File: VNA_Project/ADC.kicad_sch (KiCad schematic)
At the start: 27 parts, among them U3 AD9238BSTZ-20, U4 LT1813CS8-TRPBF, U5 LT1813CS8-TRPBF

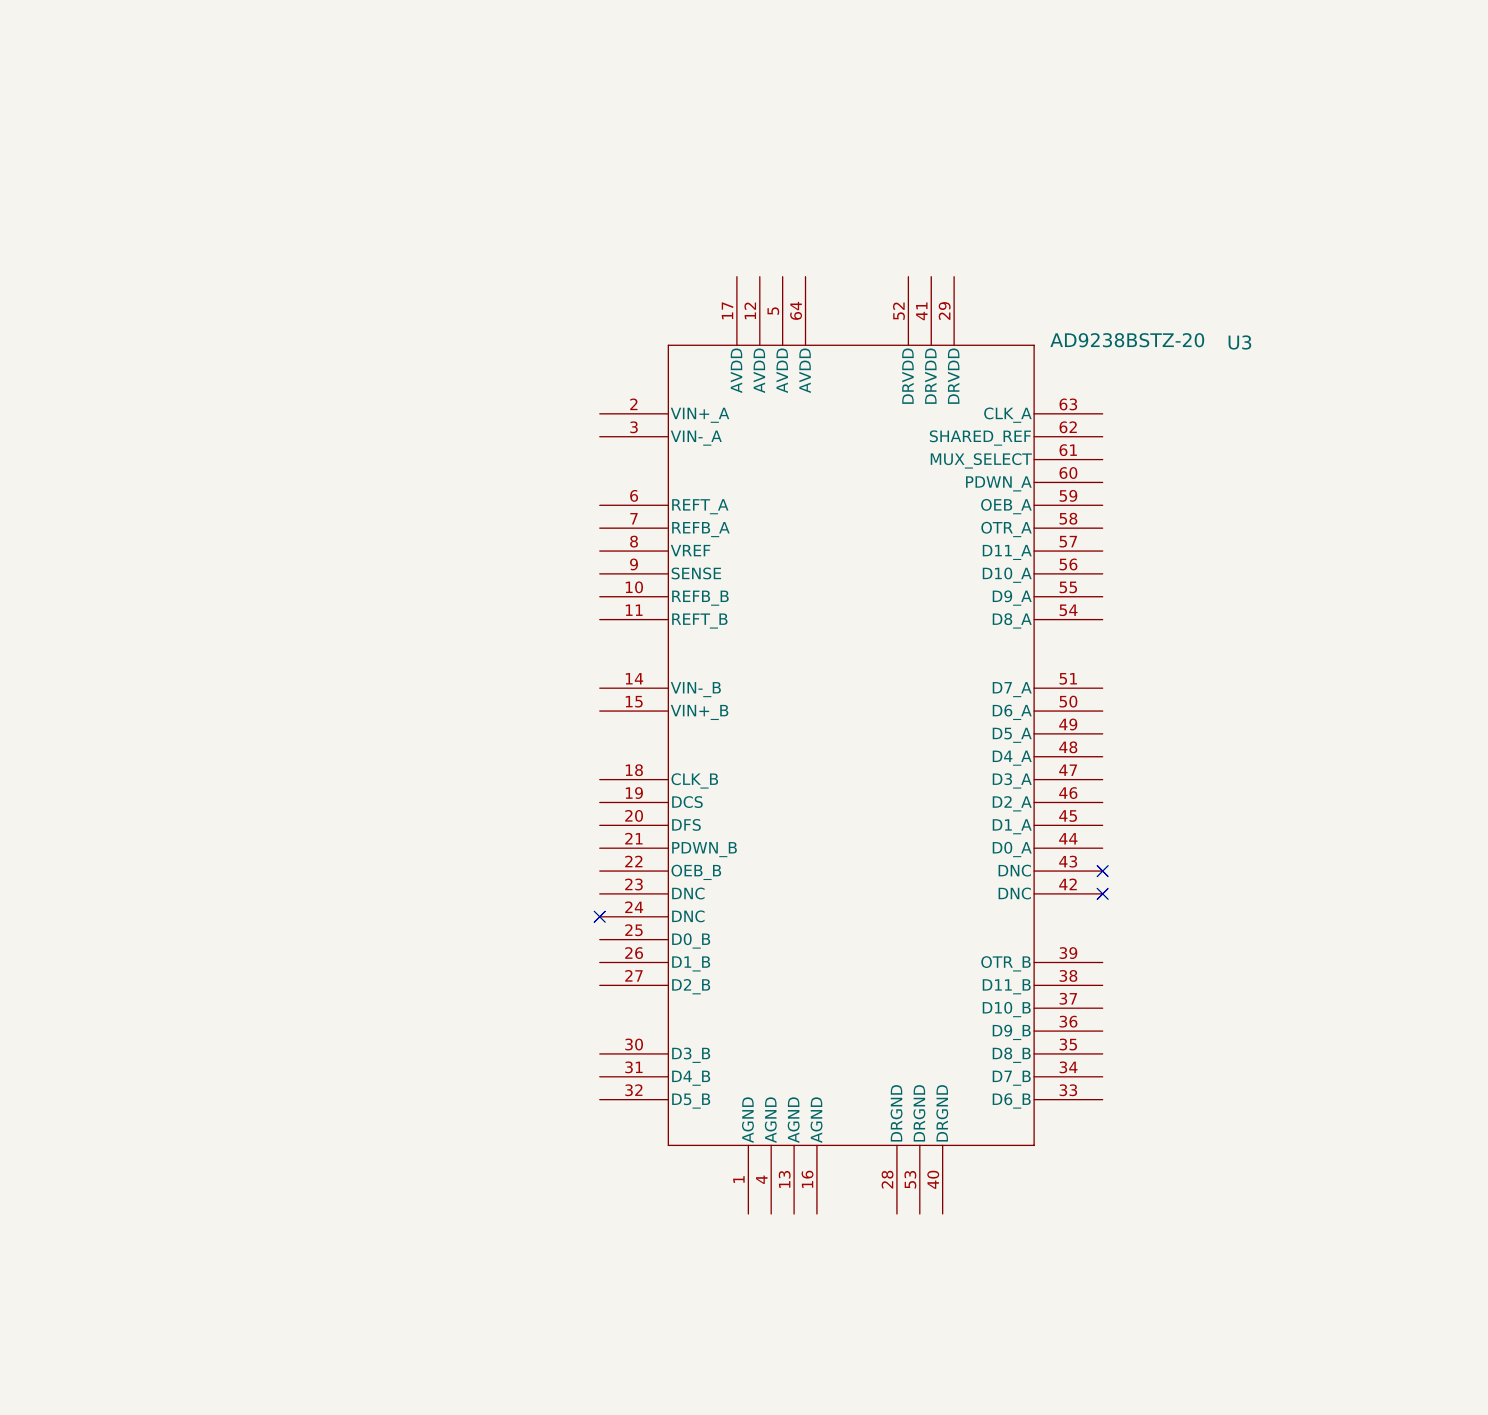
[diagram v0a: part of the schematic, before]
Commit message: adc
adc
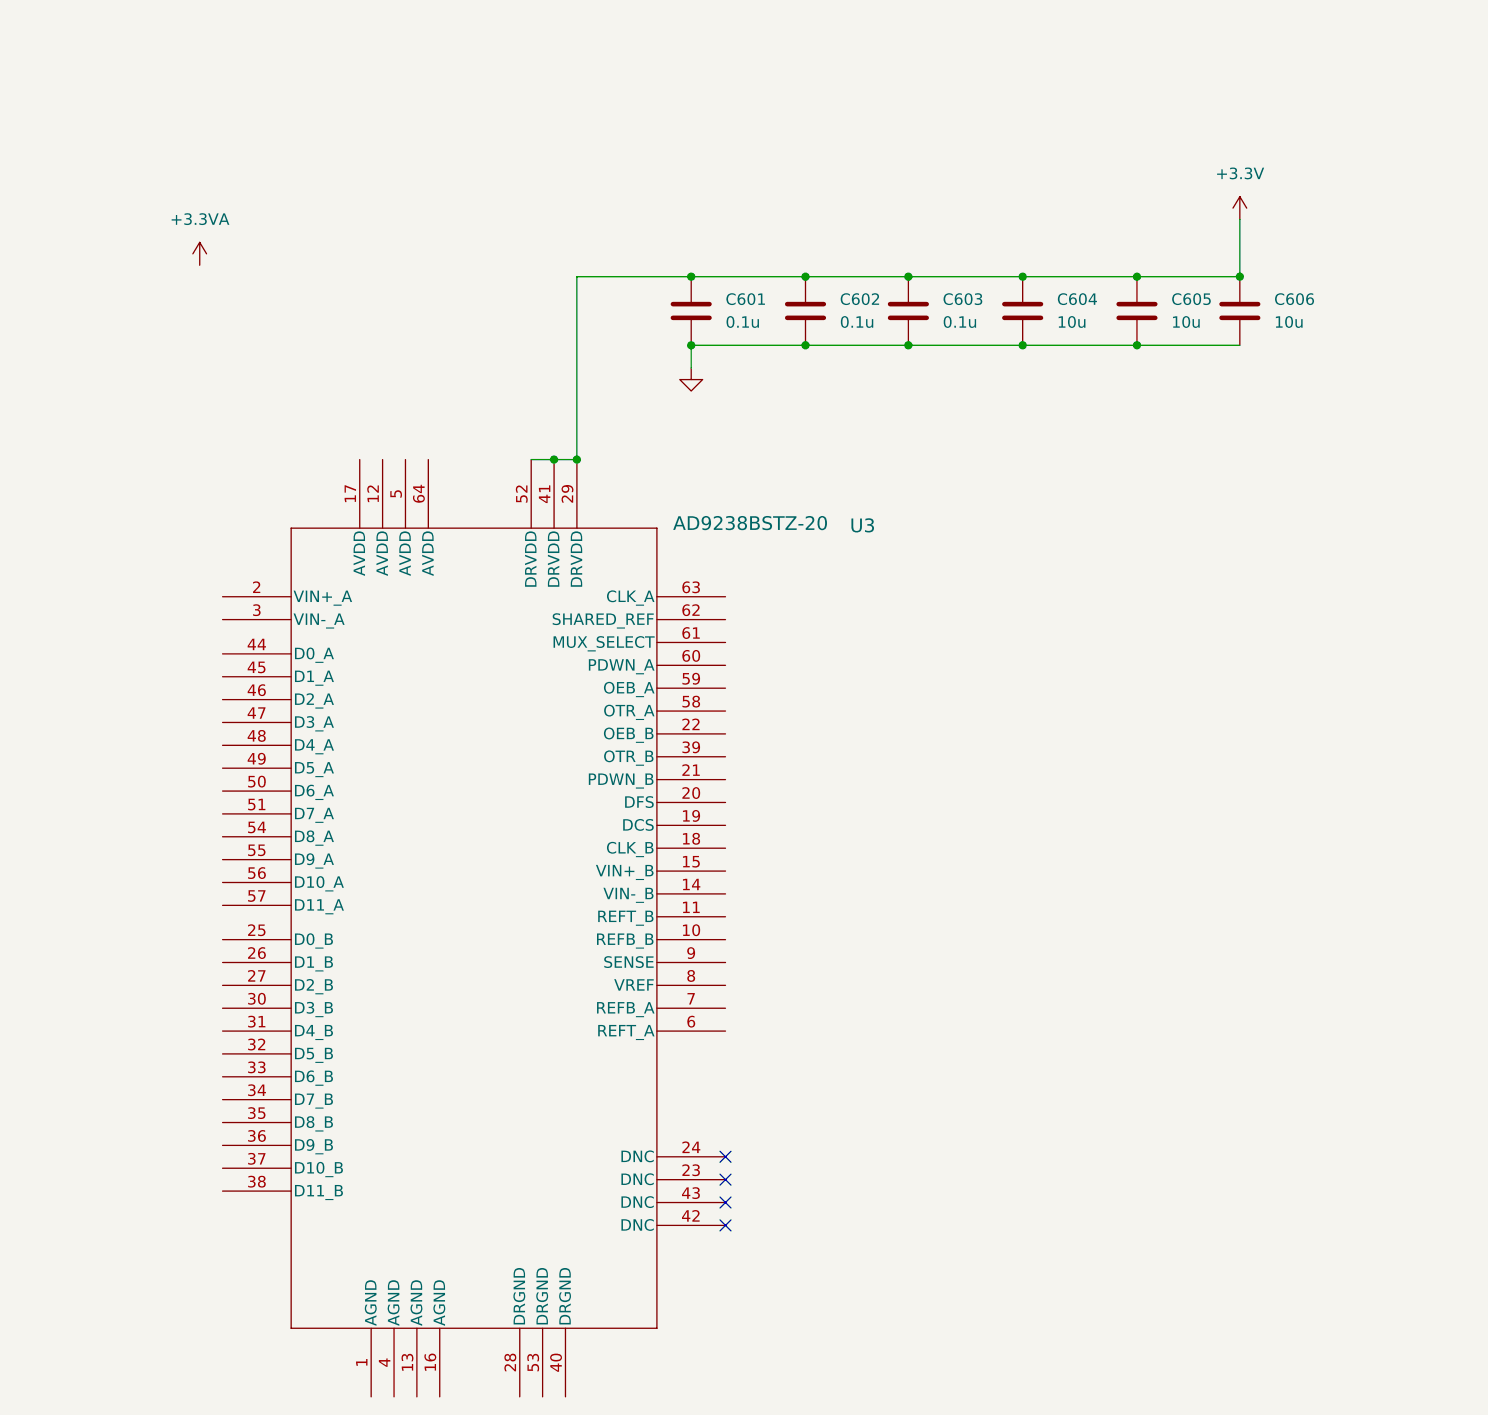
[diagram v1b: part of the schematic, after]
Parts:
- added C601, C602, C603: 0.1u, symbol Device:C
- added C604, C605, C606: 10u, symbol Device:C
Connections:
- net GND: now also C601.2, C602.2, C603.2, C604.2, C605.2, C606.2
- net +3.3V: now reaches U3.29 (DRVDD)
- net +3.3V: now also U3.41 (DRVDD), U3.52 (DRVDD), C601.1, C602.1, C603.1, C604.1, C605.1, C606.1
- no-connect marks 3 -> 4
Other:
- moved on the sheet: U3

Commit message: adc
adc
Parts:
- added C27, C28, C29, C31: 0.1u, symbol Device:C
- added C30: 10u, symbol Device:C
- added C32, C33: 100p, symbol Device:C_Small
- added FB1, FB2: FerriteBead, symbol Device:FerriteBead
- added R30, R31, R32, R33, R34, R35, R36, R37: 499, symbol Device:R_Small
- added U7, U8: AD8138ARZ, R_8_ADI, symbol Non_KiCad_Symbols:AD8138ARZ
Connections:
- net GND: now also U3.1 (AGND), U3.13 (AGND), U3.16 (AGND), U3.28 (DRGND), U3.4 (AGND), U3.40 (DRGND), U3.53 (DRGND), C27.2, C28.2, C29.2, C30.2, C31.2, C32.2, C33.2, R31.1, R34.1, U7.6 (V-), U8.6 (V-)
- net OUTA: now also R30.1
- net OUTA2: now also R37.1
- net at U3.12 (AVDD): now also U3.17 (AVDD), U3.5 (AVDD), U3.64 (AVDD), C27.1, C28.1, C29.1, C31.1, FB2.2
- net diffout2_-: now reaches U3.14 (VIN-_B)
- net diffout2_-: now also R36.2, U8.5 (-OUT)
- net diffout2_+: now reaches U3.15 (VIN+_B)
- net diffout2_+: now also R35.2, U8.4 (+OUT)
- net diffout_+: now reaches U3.2 (VIN+_A)
- net diffout_+: now also R32.2, U7.4 (+OUT)
- net D0_B: now reaches U3.25 (D0_B)
- net D1_B: now reaches U3.26 (D1_B)
- net D2_B: now reaches U3.27 (D2_B)
- net diffout_-: now reaches U3.3 (VIN-_A)
- net diffout_-: now also R33.2, U7.5 (-OUT)
- net D3_B: now reaches U3.30 (D3_B)
- net D4_B: now reaches U3.31 (D4_B)
- net D5_B: now reaches U3.32 (D5_B)
- net D6_B: now reaches U3.33 (D6_B)
- net D7_B: now reaches U3.34 (D7_B)
- net D8_B: now reaches U3.35 (D8_B)
- net D9_B: now reaches U3.36 (D9_B)
- net D10_B: now reaches U3.37 (D10_B)
- net D11_B: now reaches U3.38 (D11_B)
- net D0_A: now reaches U3.44 (D0_A)
- net D1_A: now reaches U3.45 (D1_A)
- net D2_A: now reaches U3.46 (D2_A)
- net D3_A: now reaches U3.47 (D3_A)
- net D4_A: now reaches U3.48 (D4_A)
- net D5_A: now reaches U3.49 (D5_A)
- net D6_A: now reaches U3.50 (D6_A)
- net D7_A: now reaches U3.51 (D7_A)
- net D8_A: now reaches U3.54 (D8_A)
- net D9_A: now reaches U3.55 (D9_A)
- net D10_A: now reaches U3.56 (D10_A)
- net D11_A: now reaches U3.57 (D11_A)
- net +3.3V: no longer names the net of C601.1, C602.1, C603.1, C604.1, C605.1, C606.1, U3.29 (DRVDD), U3.41 (DRVDD), U3.52 (DRVDD)
- net +3.3V: now also FB1.1
- new net: R36.1, R37.2, U8.8 (+IN)
- new net: R34.2, R35.1, U8.1 (-IN)
- new net: R31.2, R32.1, U7.1 (-IN)
- new net: R30.2, R33.1, U7.8 (+IN)
- new net +3V0: C30.1, FB1.2, FB2.1
- new net VCC: U7.3 (V+), U8.3 (V+)
- new net VREF_ADCD: C32.1, C33.1, U7.2 (VOCM), U8.2 (VOCM)
- no-connect marks 4 -> 6
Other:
- note added: "typical power dissipation of 12 mW"
- moved on the sheet: C601, C602, C603, C604, C605, C606, U3
